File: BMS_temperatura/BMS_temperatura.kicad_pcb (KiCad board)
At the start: 2 copper layers, 100.1 x 100.1 mm, 142 parts, among them J101 Conn_01x08_Male, Q101 MMBT3904, U1 UFRGS_PILL, U101 74HC4051, U103 74HC4051, U105 74HC4051, U110 MCP2558, U112 LM324, U1801 LM324, U1901 LM324, U2001 LM324, U201 LM324, U203 TL431, U2101 LM324, U2201 LM324, U2301 LM324, U301 LM317

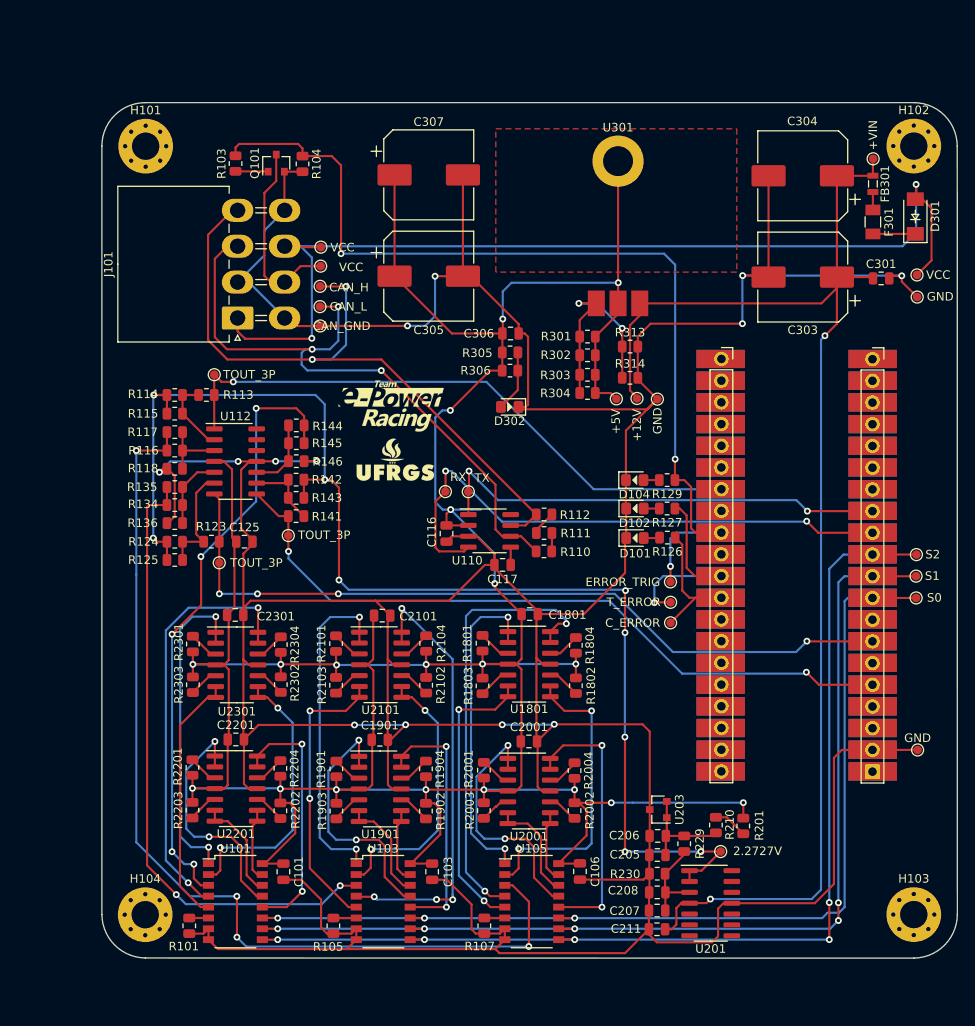
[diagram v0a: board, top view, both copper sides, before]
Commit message: layout final bms temp
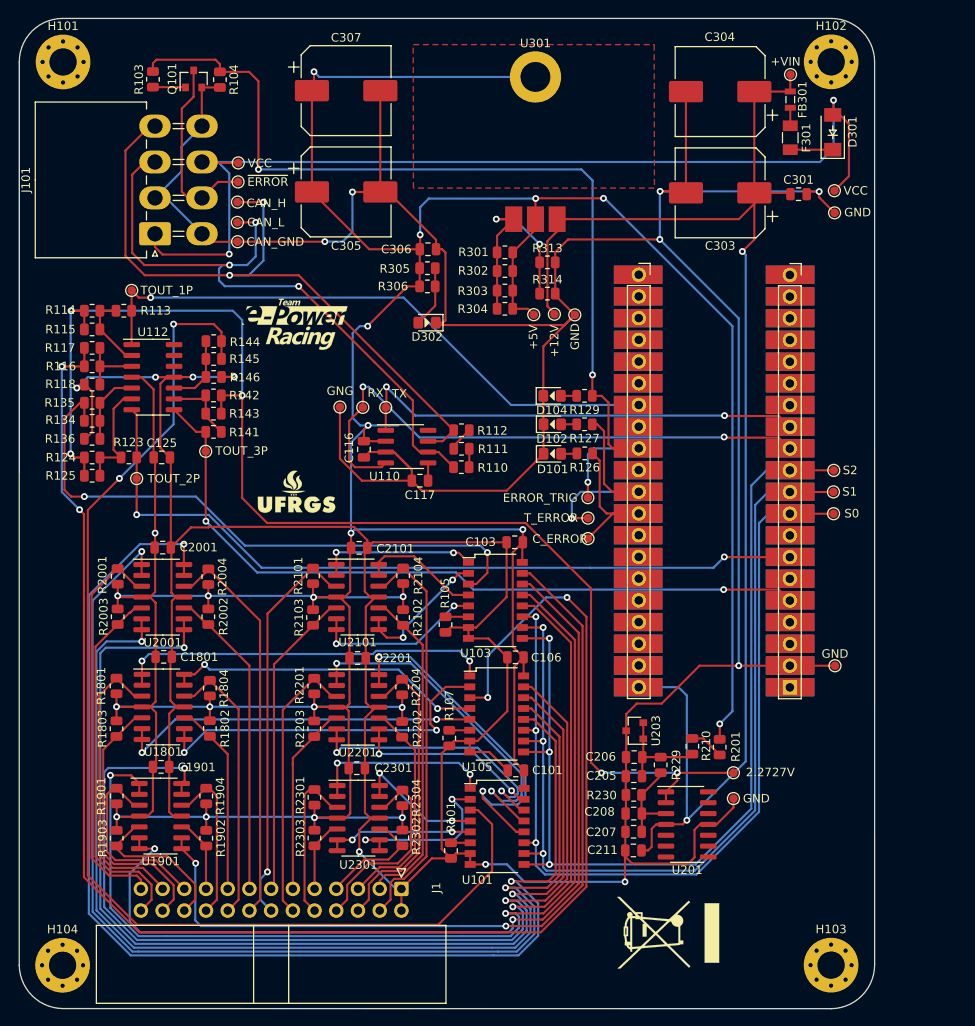
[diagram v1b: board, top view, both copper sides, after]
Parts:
- added G104: SYM_LASER_Large, Symbol:WEEE-Logo_8.4x12mm_SilkScreen, F.Cu at (137.5, 184.6)
- added J1: TEMP_IDC_26_CONN, Connector_IDC:IDC-Header_2x13_P2.54mm_Horizontal, F.Cu at (106.3, 179.5)
- added TP22: GNG, e-Power:TestPoint_Pad_D1.0mm, F.Cu at (99.1, 123.1)
- added TP29: GND, e-Power:TestPoint_Pad_D1.0mm, F.Cu at (145.2, 168.9)
- TP10: value TOUT_3P -> TOUT_1P
- TP11: value VCC -> ~ERROR
- TP2: value TOUT_3P -> TOUT_2P
- moved U2001 48.5 mm to (78.4, 145.3)
- moved C2001 48.5 mm to (78.4, 139.5)
- moved R2002 48.5 mm to (83.7, 147.6)
- moved R2004 48.5 mm to (83.7, 143.0)
- moved R2001 48.5 mm to (73.1, 142.9)
- moved R2003 48.5 mm to (73.1, 147.6)
- moved R1802 43.1 mm to (83.9, 160.7)
- moved R1804 43.1 mm to (83.9, 156.0)
- moved C1801 43.1 mm to (78.5, 152.3)
- moved R1801 43.1 mm to (73.0, 155.7)
- moved R1803 43.1 mm to (73.0, 160.7)
- moved U1801 43.1 mm to (78.4, 158.2)
- moved C103 39.7 mm to (119.6, 138.9), turned to 0 degrees
- moved R105 37.6 mm to (111.5, 148.6)
- moved U103 37.6 mm to (117.3, 145.7)
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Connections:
- U1 pad 40: Net-(U1-Pad40) -> +12V
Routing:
- net /T3: track 8.37 -> 134.3 mm, vias 0 -> 2
- net /T2: track 13.1 -> 128.3 mm, vias 0 -> 2
- net /T4: track 32.0 -> 144.0 mm
- net +5V: track 416.3 -> 527.2 mm, vias 19 -> 22
- net /T1: track 29.2 -> 138.0 mm
- net /T12: track 30.1 -> 126.6 mm
- net /T10: track 12.7 -> 107.1 mm, vias 0 -> 2
- net /T9: track 30.2 -> 119.4 mm
- net /T11: track 8.79 -> 97.9 mm, vias 0 -> 2
- net /TOUT_1: track 114.2 -> 183.2 mm
- net /TOUT_3: track 72.0 -> 138.8 mm, vias 5 -> 2
- net /Temperature Sensors/TS_16: track 3.74 -> 47.9 mm
- net /Temperature Sensors/TS_13: track 3.61 -> 46.8 mm, vias 0 -> 1
- net /Temperature Sensors/TS_1: track 3.66 -> 46.7 mm
- net /Temperature Sensors/TS_4: track 3.76 -> 46.8 mm
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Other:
- board size 100.1 x 100.1 mm -> 100.1 x 115.9 mm
